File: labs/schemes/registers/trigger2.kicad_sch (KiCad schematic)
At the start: 2 parts, among them K2 4PDT, K3 4PDT

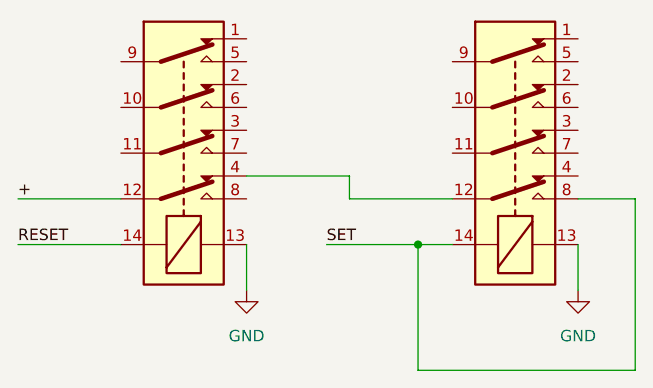
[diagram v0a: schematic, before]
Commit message: Many fixes
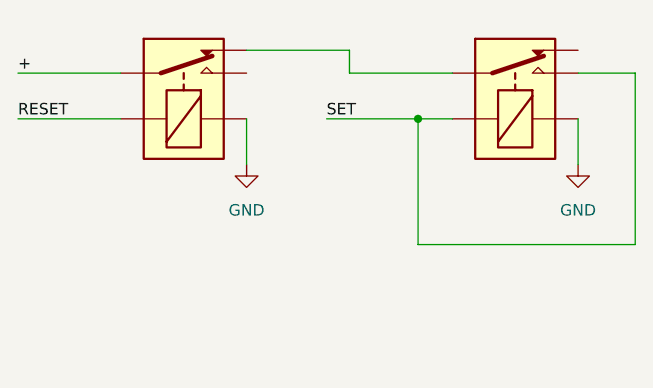
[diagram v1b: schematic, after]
